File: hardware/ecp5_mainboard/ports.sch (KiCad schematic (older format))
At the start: 93 parts, among them J3 HDMI_A, J4 USB_A, P4 JK0654219, U17 TPS2041B, U18 PCA9306, U19 TFP410, U20 TPS2041B, U21 KSZ9031RNXCA, U22 USB3300-EZK, Y2 25MHz, Y3 24MHz

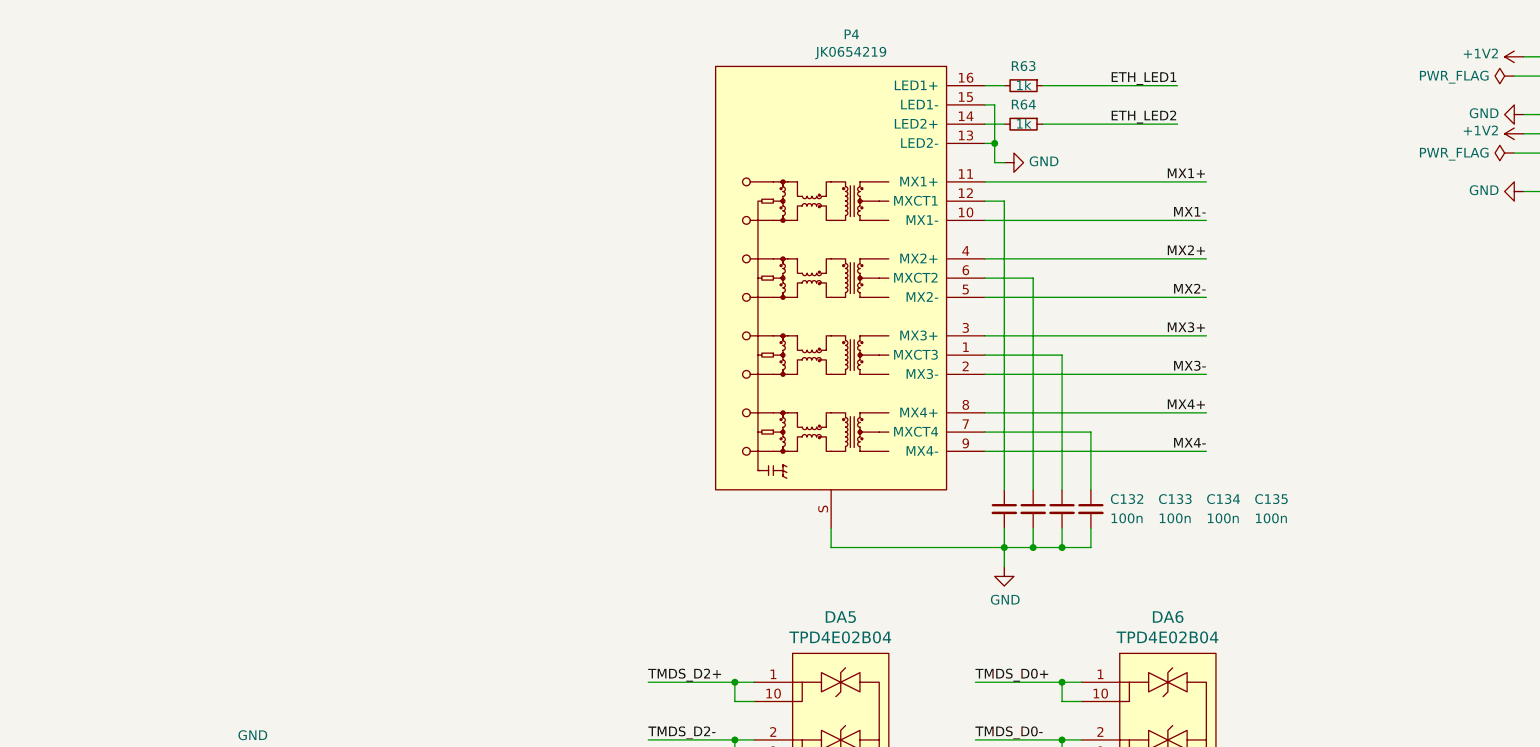
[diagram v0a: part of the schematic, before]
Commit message: hardware/mainboard: add microSD
Signed-off-by: David Shah <dave@ds0.me>
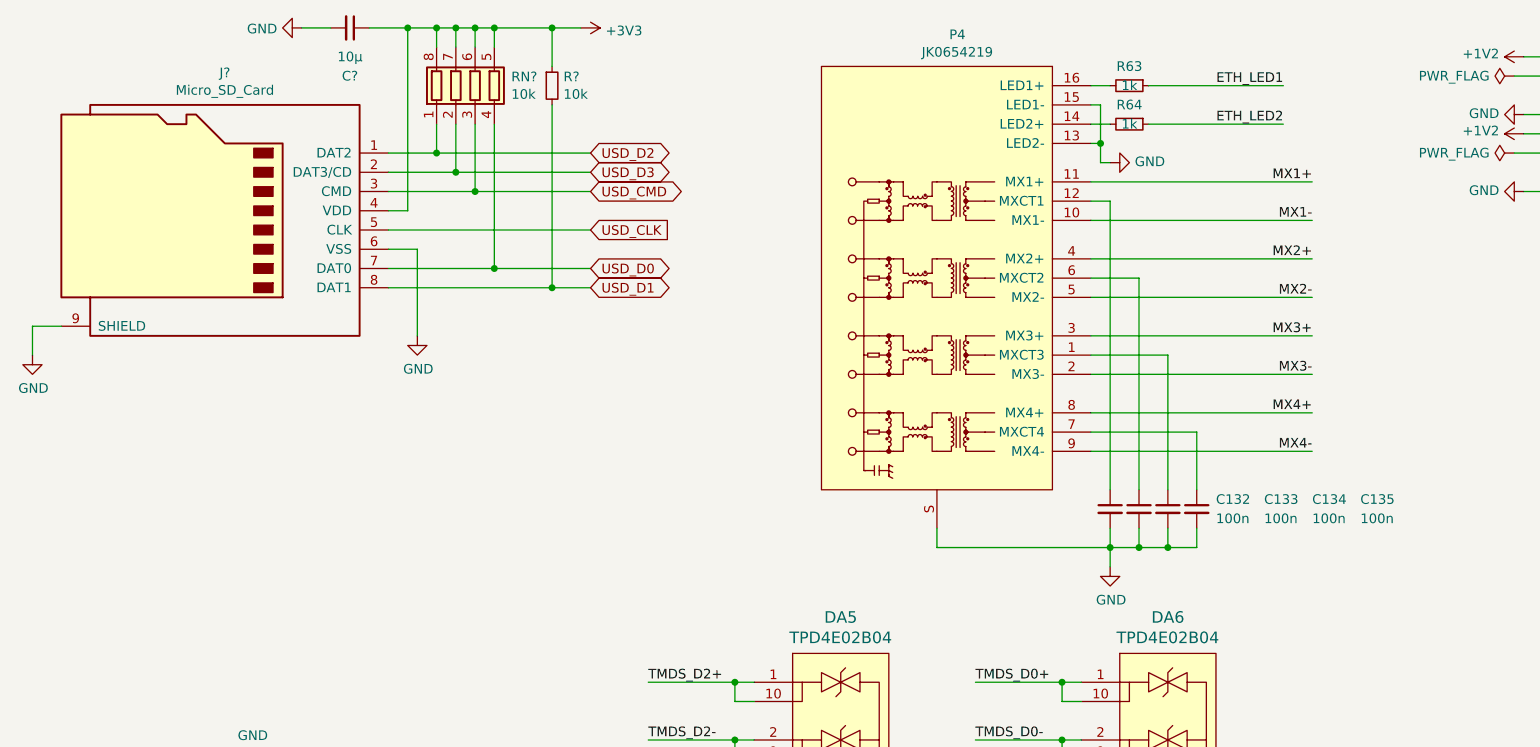
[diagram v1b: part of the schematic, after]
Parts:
- added C?: 10µ, symbol Device:C_Small
- added J?: Micro_SD_Card, symbol Connector:Micro_SD_Card
- added R?: 10k, symbol Device:R_Small
- added RN?: 10k, symbol Device:R_Pack04
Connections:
- net +3V3: now also C?.1, J?.4 (VDD), R?.1, RN?.5 (R4.2), RN?.6 (R3.2), RN?.7 (R2.2), RN?.8 (R1.2)
- net GND: now also C?.2, J?.6 (VSS), J?.9 (SHIELD)
- new net USD_CLK: J?.5 (CLK)
- new net USD_CMD: J?.3 (CMD), RN?.3 (R3.1)
- new net USD_D0: J?.7 (DAT0), RN?.4 (R4.1)
- new net USD_D1: J?.8 (DAT1), R?.2
- new net USD_D2: J?.1 (DAT2), RN?.1 (R1.1)
- new net USD_D3: J?.2 (DAT3/CD), RN?.2 (R2.1)
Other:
- moved on the sheet: C132, C133, C134, C135, P4, R63, R64
